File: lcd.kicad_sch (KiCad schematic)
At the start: 11 parts, among them J1 FPC-05F-12PH20, Q2 SS8050

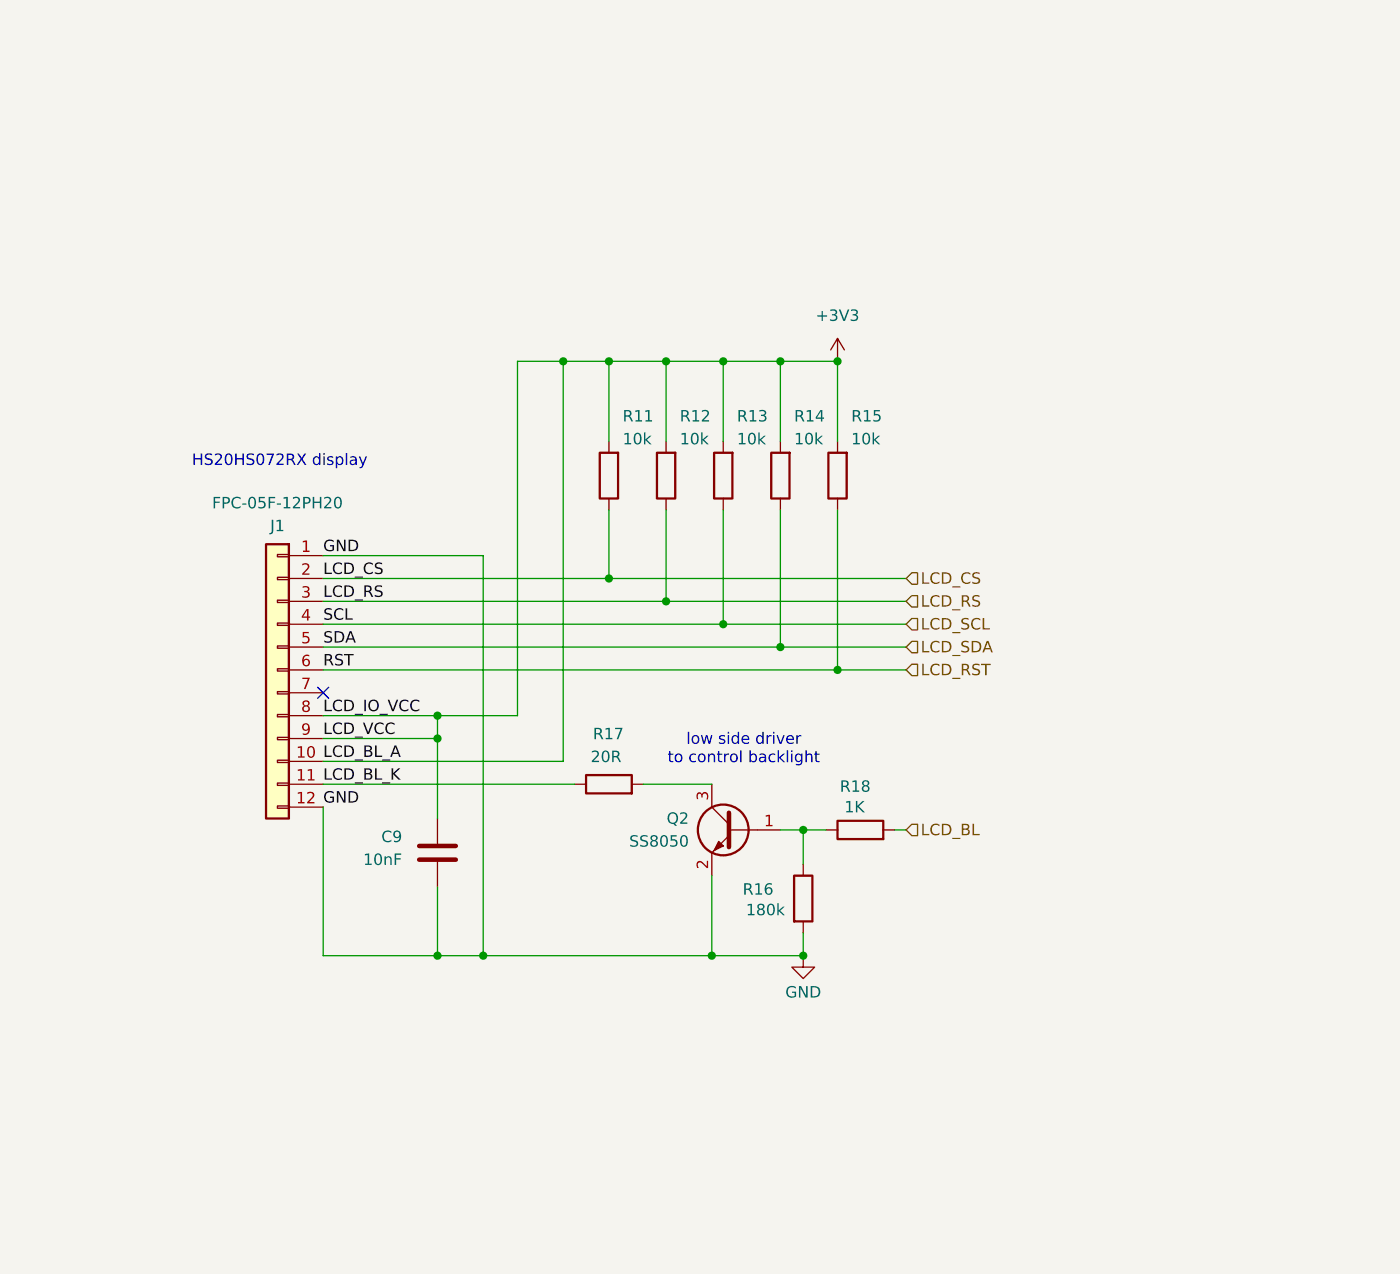
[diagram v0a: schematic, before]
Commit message: remove backups, removed old chip
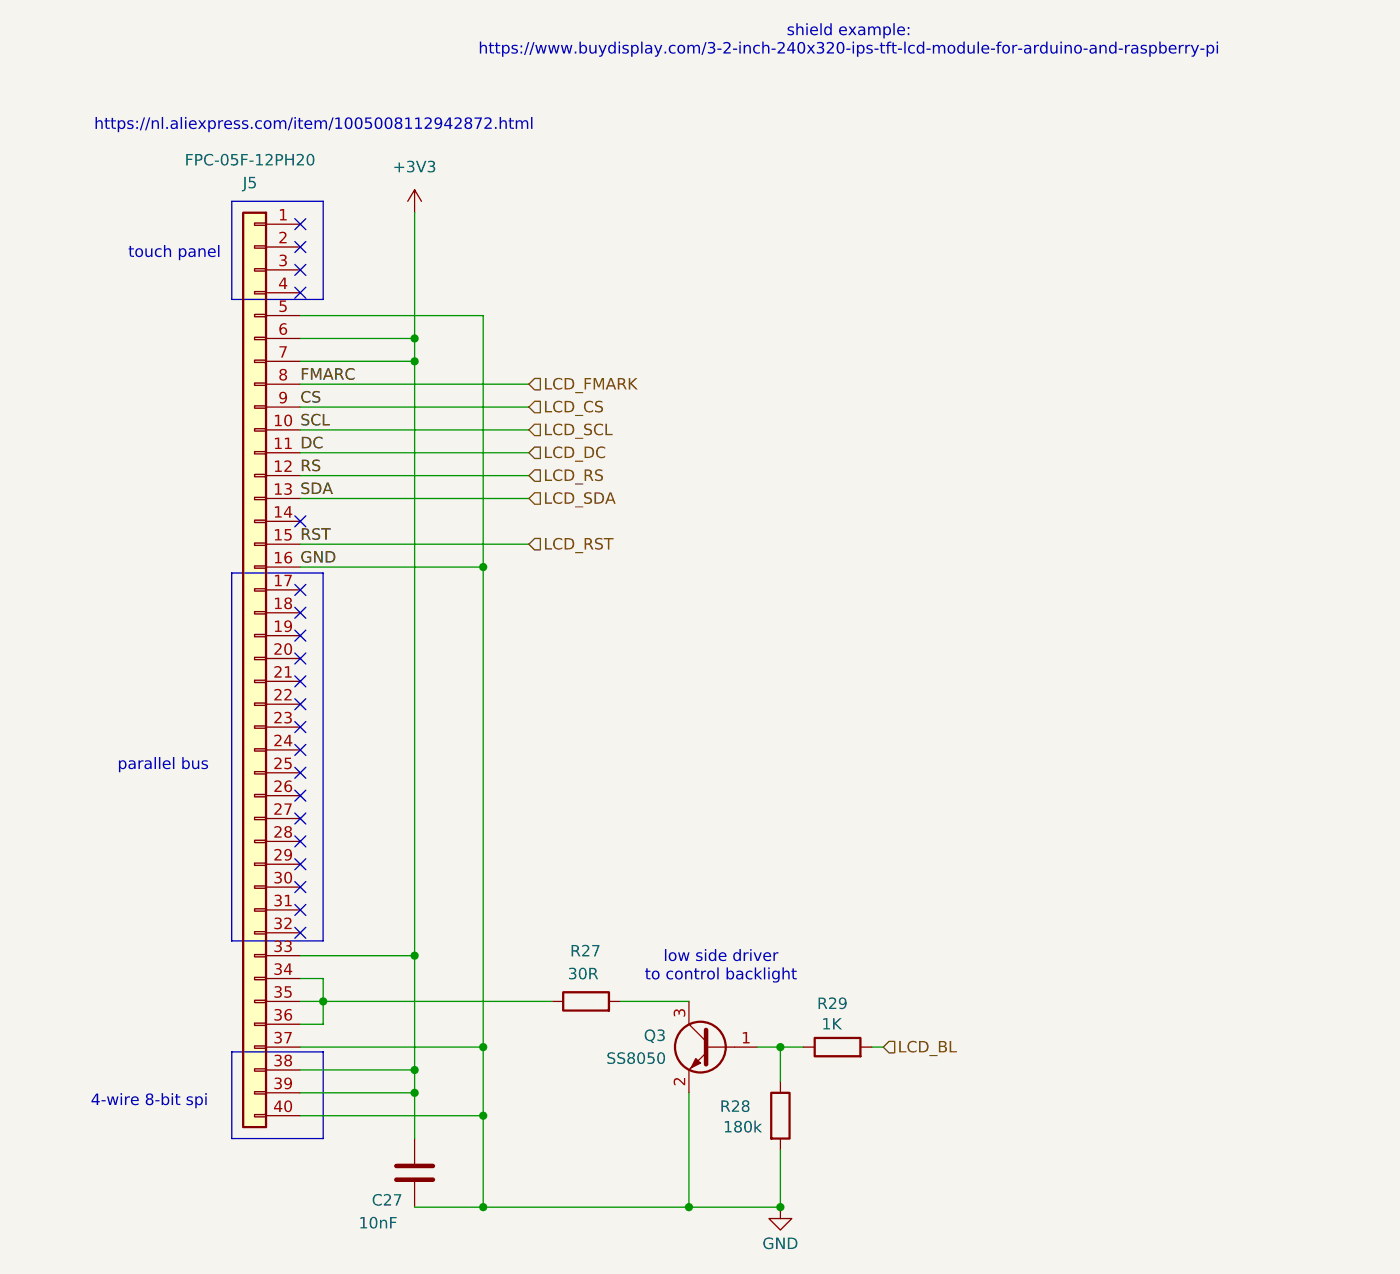
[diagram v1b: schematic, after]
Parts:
- removed C9: 10nF, Capacitor_SMD:C_0603_1608Metric, symbol Device:C
- removed J1: FPC-05F-12PH20, Connector_FFC-FPC:TE_1-1734839-2_1x12-1MP_P0.5mm_Horizontal, symbol Connector_Generic:Conn_01x12
- removed Q2: SS8050, Package_TO_SOT_SMD:SOT-23, symbol Transistor_BJT:SS8050
- removed R11, R12, R13, R14, R15: 10k, Resistor_SMD:R_0603_1608Metric, symbol Device:R
- removed R16: 180k, Resistor_SMD:R_0603_1608Metric, symbol Device:R
- removed R17: 20R, Resistor_SMD:R_0603_1608Metric, symbol Device:R
- removed R18: 1K, Resistor_SMD:R_0603_1608Metric, symbol Device:R
- added C27: 10nF, Capacitor_SMD:C_0603_1608Metric, symbol Device:C
- added J5: FPC-05F-12PH20, Connector_FFC-FPC:TE_4-1734839-0_1x40-1MP_P0.5mm_Horizontal, symbol Connector_Generic:Conn_01x40
- added Q3: SS8050, Package_TO_SOT_SMD:SOT-23, symbol Transistor_BJT:SS8050
- added R27: 30R, Resistor_SMD:R_0603_1608Metric, symbol Device:R
- added R28: 180k, Resistor_SMD:R_0603_1608Metric, symbol Device:R
- added R29: 1K, Resistor_SMD:R_0603_1608Metric, symbol Device:R
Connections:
- net +3V3: now also C27.2, J5.33 (Pin_33), J5.38 (Pin_38), J5.39 (Pin_39), J5.6 (Pin_6), J5.7 (Pin_7)
- net GND: now also C27.1, J5.16 (Pin_16), J5.37 (Pin_37), J5.40 (Pin_40), J5.5 (Pin_5), Q3.2 (E), R28.2
- net LCD_BL: now also R29.2
- net LCD_CS: now also J5.9 (Pin_9)
- net LCD_RS: now also J5.12 (Pin_12)
- net LCD_RST: now also J5.15 (Pin_15)
- net LCD_SCL: now also J5.10 (Pin_10)
- net LCD_SDA: now also J5.13 (Pin_13)
- new net: Q3.1 (B), R28.1, R29.1
- new net: Q3.3 (C), R27.2
- new net: J5.34 (Pin_34), J5.35 (Pin_35), J5.36 (Pin_36), R27.1
- new net LCD_DC: J5.11 (Pin_11)
- new net LCD_FMARK: J5.8 (Pin_8)
- no-connect marks 1 -> 21
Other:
- note added: "4-wire 8-bit spi"
- note added: "https://nl.aliexpress.com/item/1005008112942872.html"
- note added: "parallel bus"
- note added: "shield example: https://www.buydisplay.com/3-2-inch-240x320-ips-tft-lcd-module-for-arduino-and-raspberry-pi"
- note added: "touch panel"
- note removed: "HS20HS072RX display"
